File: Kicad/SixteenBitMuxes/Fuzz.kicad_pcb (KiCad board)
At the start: 2 copper layers, 100 x 82 mm, 110 parts, among them J1 Audio In/Out JST XH, J10 Key Pad JST XH, J11 LCD JST XH, J12 Bypass Switch JST XH, J2 POT B10K JST XH, J3 POT B5K JST XH, J4 VOL POT A100K JST XH, J5 PowerTest_PinHeader, J6 9V Power JST XH, J7 Boot Reset PinHeader, J9 SWD_PinHeader, Q1 PN2222A, Q10 2SC1815, Q11 PN2222A, Q12 S9013, Q13 MMBT3904, Q14 S9018, Q15 BC848B, Q16 2SC1623, Q17 MPSA18, Q18 MMBT5551L, Q19 2N5088, Q2 MMBT3904, Q20 MMBTA42, Q21 BC807, Q22 BC846, Q23 BC847B, Q24 BC847C, Q25 BC848B, Q26 S9013, Q27 S9018, Q28 C945, Q29 2SC1623, Q3 MMBT5551L, Q30 2SC1815, Q31 MPSA18, Q32 2N5088, Q4 MMBTA42, Q5 BC807, Q6 BC846, Q7 BC847B, Q8 BC847C, Q9 C945, U1 AMS1117-5.0, U2 AMS1117-3.3, U21 CD4051B, U22 4504, U23 4504, U24 4504, U25 CD4053B, U3 STM32F103C8Tx, U4 CD4051B, U6 CD4067BM, U7 CD4067BM, U8 CD4067BM, U9 CD4067BM, Y1 8MHz

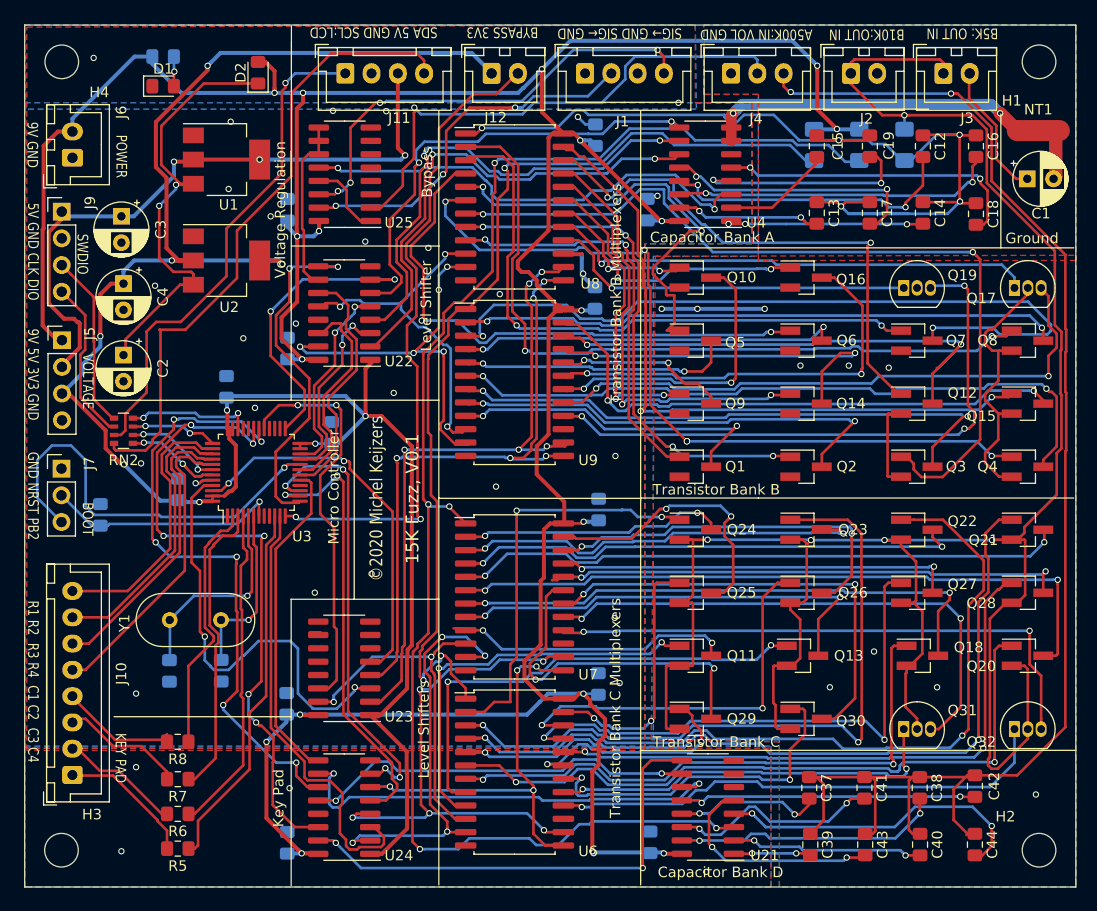
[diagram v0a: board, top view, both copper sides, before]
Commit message: PCB mostly
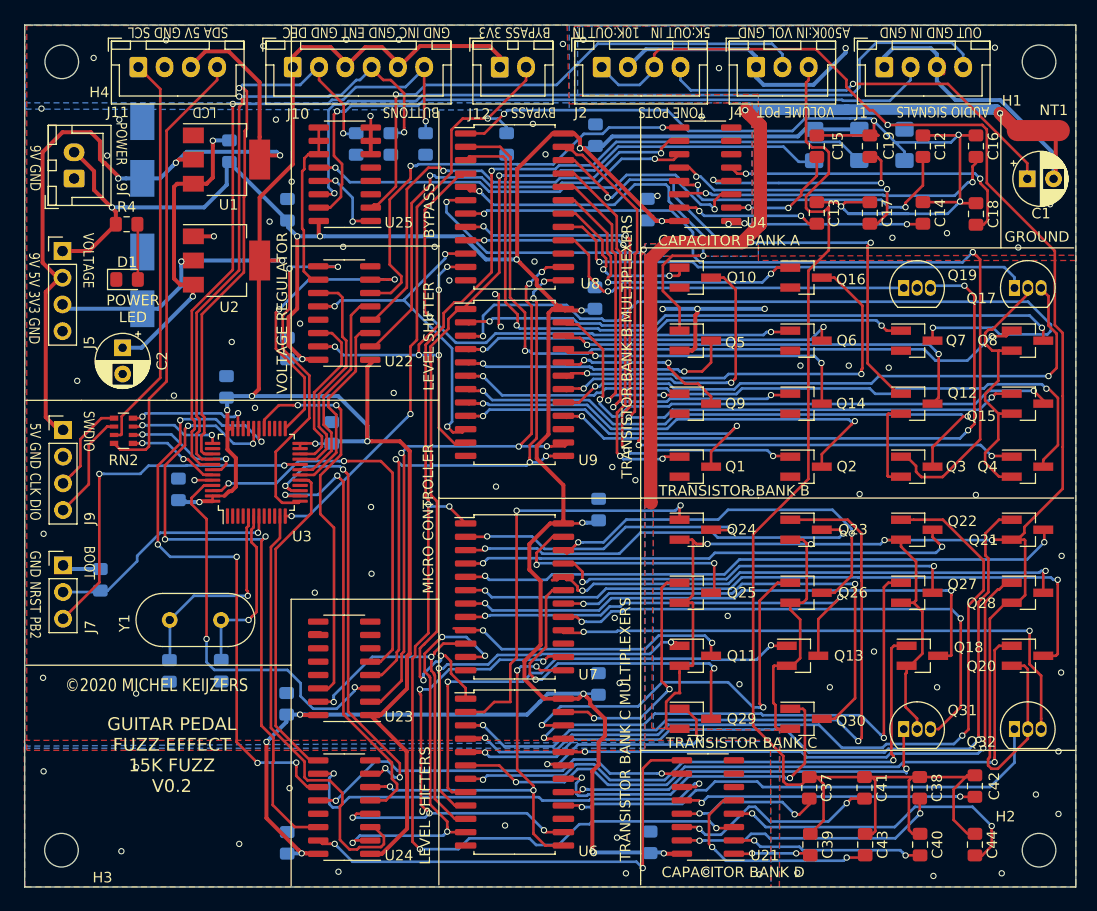
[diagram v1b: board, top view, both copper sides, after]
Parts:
- removed J3: POT B5K JST XH, Connector_JST:JST_XH_B2B-XH-A_1x02_P2.50mm_Vertical
- removed REF**: KiCad-Logo2_30mm_SilkScreen, Symbol:KiCad-Logo2_30mm_SilkScreen
- C3, C4: footprint Capacitor_THT:CP_Radial_D5.0mm_P2.50mm -> Diode_SMD:D_SMB_Handsoldering; moved to B.Cu
- D2: moved to B.Cu
- J10: value Key Pad JST XH -> JST XH Buttons; footprint Connector_JST:JST_XH_B8B-XH-A_1x08_P2.50mm_Vertical -> Connector_JST:JST_XH_B6B-XH-A_1x06_P2.50mm_Vertical
- J2: value POT B10K JST XH -> TONE_POTS; footprint Connector_JST:JST_XH_B2B-XH-A_1x02_P2.50mm_Vertical -> Connector_JST:JST_XH_B4B-XH-A_1x04_P2.50mm_Vertical
- R4: moved to F.Cu
- R5, R6, R7, R8: value 1K -> 10K; moved to B.Cu
- moved J10 70.5 mm to (55.5, 34.0), turned to 0 degrees
- moved R5 69.1 mm to (61.5, 41.3), turned to 270 degrees
- moved R6 66.9 mm to (64.8, 41.3), turned to 270 degrees
- moved R8 64.9 mm to (75.8, 41.3), turned to 90 degrees
- moved R7 64.9 mm to (68.1, 41.3), turned to 270 degrees
- moved J1 28.5 mm to (111.8, 34.0)
- moved J2 23.7 mm to (84.9, 34.0)
- moved J9 20.8 mm to (33.6, 68.5)
- moved J11 19.7 mm to (40.8, 34.0)
- moved D1 18.7 mm to (39.7, 54.2)
- moved R4 16.3 mm to (39.7, 49.0)
- moved J7 9.20 mm to (33.6, 81.4)
- moved J5 8.48 mm to (33.6, 51.5)
- moved D2 7.95 mm to (49.5, 42.0), turned to 270 degrees
- moved C3 6.62 mm to (41.2, 41.9), turned to 90 degrees
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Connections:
- J1 pad 1: GND -> GNDA
- J1 pad 3: GND -> GNDA
- J10 pad 1: Net-(J10-Pad1) -> +3V3
- J10 pad 2: Net-(J10-Pad2) -> /Mcu/GPIO_BUTTON_DECREASE
- J10 pad 3: Net-(J10-Pad3) -> +3V3
- J10 pad 4: Net-(J10-Pad4) -> /Mcu/GPIO_BUTTON_ENTER
- J10 pad 5: /Mcu/GPIO_KEYPAD_ROW_4 -> +3V3
- J10 pad 6: /Mcu/GPIO_KEYPAD_ROW_3 -> /Mcu/GPIO_BUTTON_INCREASE
- J2 pad 1: /TransistorsC/EMITTER -> /B10K
- Q11 pad 2: /TransistorsC/EMITTER -> /B10K
- Q13 pad 2: /TransistorsC/EMITTER -> /B10K
- Q18 pad 2: /TransistorsC/EMITTER -> /B10K
- Q20 pad 2: /TransistorsC/EMITTER -> /B10K
- Q21 pad 2: /TransistorsC/EMITTER -> /B10K
- Q22 pad 2: /TransistorsC/EMITTER -> /B10K
- Q23 pad 2: /TransistorsC/EMITTER -> /B10K
- Q24 pad 2: /TransistorsC/EMITTER -> /B10K
- Q25 pad 2: /TransistorsC/EMITTER -> /B10K
- Q26 pad 2: /TransistorsC/EMITTER -> /B10K
- Q27 pad 2: /TransistorsC/EMITTER -> /B10K
- Q28 pad 2: /TransistorsC/EMITTER -> /B10K
- Q29 pad 2: /TransistorsC/EMITTER -> /B10K
- Q30 pad 2: /TransistorsC/EMITTER -> /B10K
- Q31 pad 2: /TransistorsC/EMITTER -> /B10K
- Q32 pad 2: /TransistorsC/EMITTER -> /B10K
- R2 pad 1: /TransistorsC/EMITTER -> /B10K
- R5 pad 1: /Mcu/GPIO_KEYPAD_COLUMN_1 -> /Mcu/GPIO_BUTTON_DECREASE
- R5 pad 2: Net-(J10-Pad1) -> GND
- R6 pad 1: /Mcu/GPIO_KEYPAD_COLUMN_2 -> /Mcu/GPIO_BUTTON_ENTER
- R6 pad 2: Net-(J10-Pad2) -> GND
- R7 pad 1: /Mcu/GPIO_KEYPAD_COLUMN_3 -> /Mcu/GPIO_BUTTON_INCREASE
- R7 pad 2: Net-(J10-Pad3) -> GND
- R8 pad 1: /Mcu/GPIO_KEYPAD_COLUMN_4 -> GND
- R8 pad 2: Net-(J10-Pad4) -> /Mcu/BYPASS_SWITCH_3V3
- U22 pad 11: /TRANSISTOR_B_SELECTION_0_3V3 -> /CAPACITOR_A_SELECTION_0_3V3
- U22 pad 14: /TRANSISTOR_B_SELECTION_1_3V3 -> /CAPACITOR_A_SELECTION_1_3V3
- U22 pad 3: /CAPACITOR_A_SELECTION_0_3V3 -> /TRANSISTOR_B_SELECTION_0_3V3
- U22 pad 5: /CAPACITOR_A_SELECTION_1_3V3 -> /TRANSISTOR_B_SELECTION_1_3V3
- U3 pad 10: /Mcu/GPIO_KEYPAD_COLUMN_1 -> Net-(U3-Pad10)
- U3 pad 2: /Mcu/GPIO_KEYPAD_COLUMN_4 -> Net-(U3-Pad2)
- U3 pad 3: /Mcu/GPIO_KEYPAD_COLUMN_3 -> Net-(U3-Pad3)
- U3 pad 38: /Mcu/GPIO_KEYPAD_ROW_1 -> Net-(U3-Pad38)
- U3 pad 39: /Mcu/GPIO_KEYPAD_ROW_2 -> /Mcu/GPIO_BUTTON_DECREASE
- U3 pad 4: /Mcu/GPIO_KEYPAD_COLUMN_2 -> Net-(U3-Pad4)
- U3 pad 40: /Mcu/GPIO_KEYPAD_ROW_3 -> /Mcu/GPIO_BUTTON_ENTER
- U3 pad 41: /Mcu/GPIO_KEYPAD_ROW_4 -> /Mcu/GPIO_BUTTON_INCREASE
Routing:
- net /B10K: track 0.00 -> 231.3 mm, vias 0 -> 5
- net /TransistorsC/EMITTER: track 216.9 -> 0.00 mm, vias 5 -> 0
- net /Mcu/GPIO_BUTTON_INCREASE: track 0.00 -> 63.7 mm, vias 0 -> 2
- net /Mcu/GPIO_BUTTON_ENTER: track 0.00 -> 60.8 mm, vias 0 -> 2
- net GNDA: track 50.5 -> 107.2 mm, vias 10 -> 30
- net +9V: track 331.0 -> 274.4 mm, vias 18 -> 15
- net /Mcu/GPIO_BUTTON_DECREASE: track 0.00 -> 55.2 mm, vias 0 -> 2
- net GND: track 41.9 -> 89.0 mm, vias 33 -> 55
- net /Mcu/GPIO_KEYPAD_COLUMN_1: track 35.4 -> 0.00 mm
- net /AudioInOut/JACK_IN_SIGNAL: track 35.4 -> 68.3 mm, vias 3 -> 1
- net /AudioInOut/JACK_OUT_SIGNAL: track 43.4 -> 75.9 mm, vias 4 -> 1
- net /Mcu/GPIO_KEYPAD_COLUMN_2: track 31.4 -> 0.00 mm
- net /Mcu/GPIO_KEYPAD_ROW_4: track 29.3 -> 0.00 mm
- net /Mcu/GPIO_KEYPAD_COLUMN_3: track 28.6 -> 0.00 mm
- net /Mcu/GPIO_KEYPAD_ROW_3: track 27.5 -> 0.00 mm
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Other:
- board text added: "10K:OUT IN"
- board text added: "5K:OUT IN"
- board text added: "AUDIO SIGNALS"
- board text added: "BUTTONS"
- board text added: "BYPASS"
- board text added: "CAPACITOR BANK A"
- board text added: "CAPACITOR BANK D"
- board text added: "FUZZ"
- board text added: "GND INC GND ENT GND DEC"
- board text added: "GROUND"
- board text added: "GUITAR PEDAL FUZZ EFFECT 15K FUZZ V0.2"
- board text added: "LCD"
- board text added: "LEVEL SHIFTER"
- board text added: "LEVEL SHIFTERS"
- board text added: "MICRO CONTROLLER"
- board text added: "OSCILLATOR CAPACITORS"
- board text added: "OUT GND IN GND"
- board text added: "POWER LED"
- board text added: "SDA 5V GND SCL"
- board text added: "TONE POTS"
- board text added: "TRANSISTOR BANK B"
- board text added: "TRANSISTOR BANK B MULTIPLEXERS"
- board text added: "TRANSISTOR BANK C"
- board text added: "TRANSISTOR BANK C MULTIPLEXERS"
- board text added: "VOLTAGE REGULATOR"
- board text added: "VOLTAGE REGULATOR DIODES"
- board text added: "VOLUME POT"
- board text added: "©2020 MICHEL KEIJZERS"
- board text removed: "15K Fuzz, V0.1"
- board text removed: "B10K:OUT IN"
- board text removed: "B5K: OUT IN"
- board text removed: "Bypass"
- board text removed: "Capacitor Bank A"
- board text removed: "Capacitor Bank D"
- board text removed: "Fuzz"
- board text removed: "Ground"
- board text removed: "KEY PAD"
- board text removed: "Key Pad"
- board text removed: "Level Shifter"
- board text removed: "Level Shifters"
- board text removed: "Micro Controller"
- board text removed: "R1 R2 R3 R4 C1 C2 C3 C4"
- board text removed: "SDA 5V GND SCL:LCD"
- board text removed: "SIG→ GND SIG← GND"
- board text removed: "Transistor Bank B"
- board text removed: "Transistor Bank B Multiplexers"
- board text removed: "Transistor Bank C"
- board text removed: "Transistor Bank C Multiplexers"
- board text removed: "Voltage Regulation"
- board text removed: "©2020 Michel Keijzers"
